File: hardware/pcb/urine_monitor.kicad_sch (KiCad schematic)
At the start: 26 parts, among them J1 LoadCell, J2 EInk_FPC, J3 USB-C_Power, Q1 SI2301, Q2 2N7002, SW1 USER_BTN, U1 RAK3172, U2 HX711, U3 TPS61220, U4 MIC5504-3.3

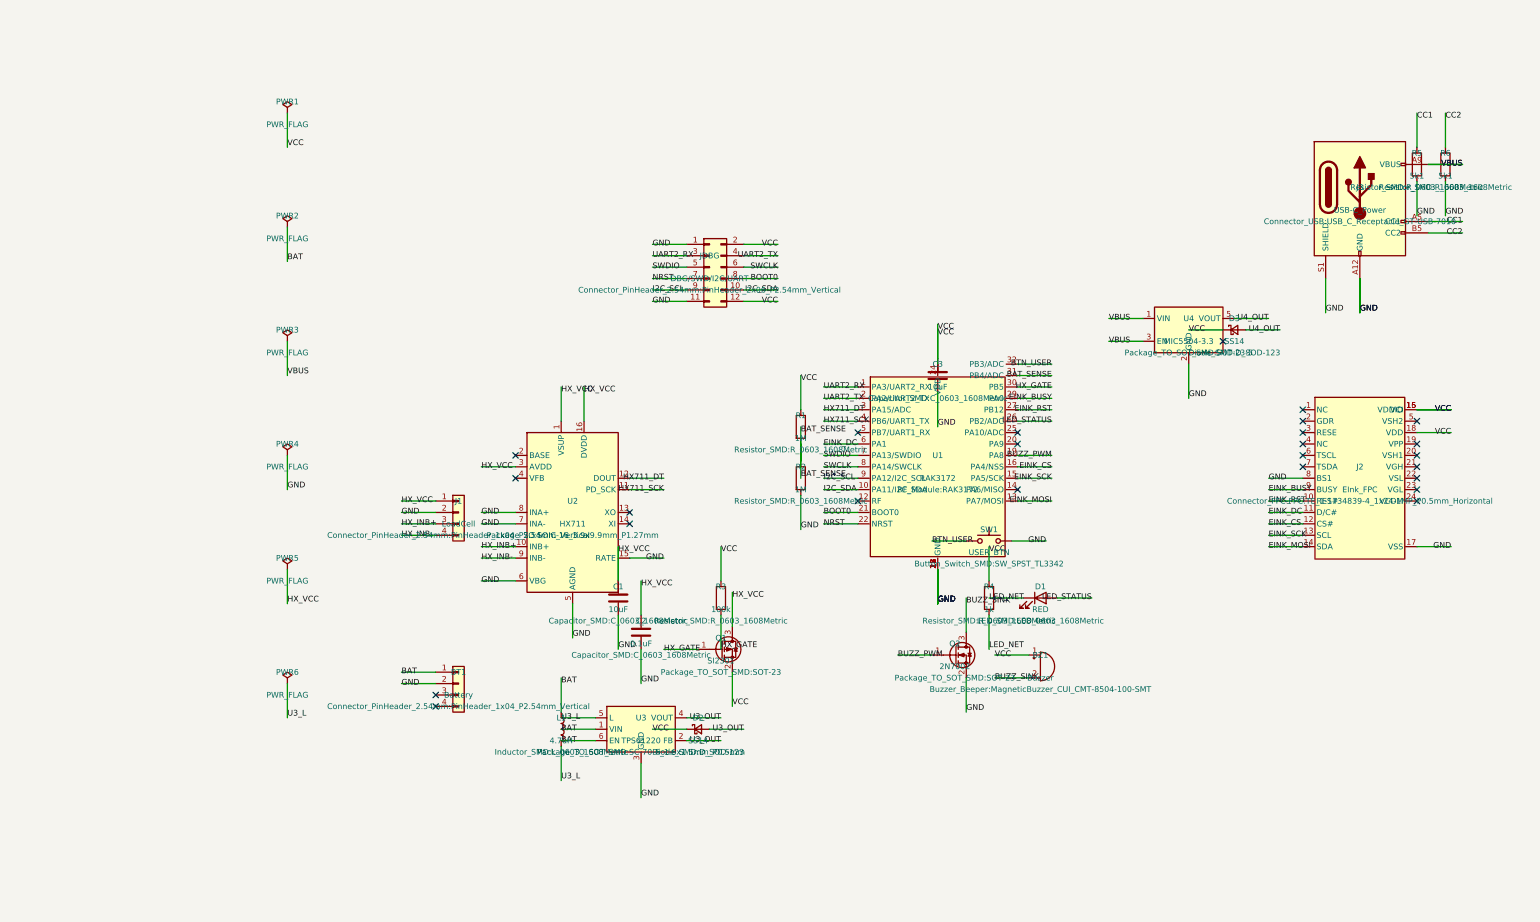
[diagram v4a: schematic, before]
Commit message: init
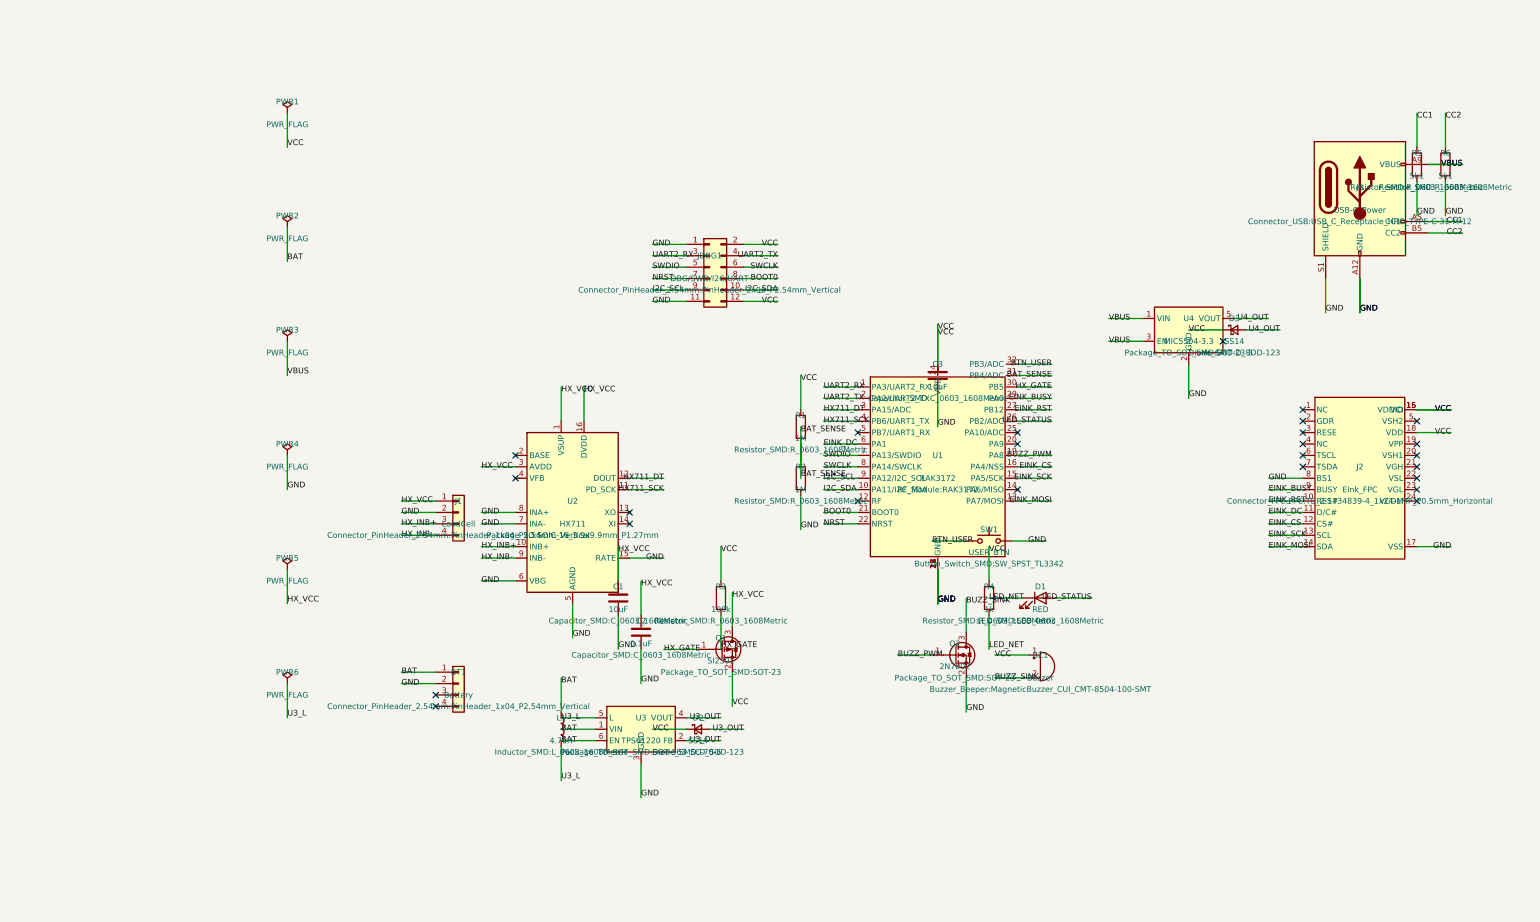
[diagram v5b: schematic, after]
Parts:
- removed JDBG: DBG/SWD/I2C/UART, Connector_PinHeader_2.54mm:PinHeader_2x06_P2.54mm_Vertical, symbol Connector_Generic:Conn_02x06_Odd_Even
- added JDBG1: DBG/SWD/I2C/UART, Connector_PinHeader_2.54mm:PinHeader_2x06_P2.54mm_Vertical, symbol Connector_Generic:Conn_02x06_Odd_Even
- J2: footprint Connector_FFC-FPC:TE_1-1734839-4_1x24-1MP_P0.5mm_Horizontal -> Connector_FFC-FPC:TE_2-1734839-4_1x24-1MP_P0.5mm_Horizontal
- J3: footprint Connector_USB:USB_C_Receptacle_GT-USB-7010 -> Connector_USB:USB_C_Receptacle_HRO_TYPE-C-31-M-12
- U3: footprint Package_TO_SOT_SMD:SC-70-6_1.6x1.5mm_P0.5mm -> Package_TO_SOT_SMD:SOT-363_SC-70-6
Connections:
- net BOOT0: now also JDBG1.8 (Pin_8)
- net GND: now also JDBG1.1 (Pin_1), JDBG1.11 (Pin_11)
- net I2C_SCL: now also JDBG1.9 (Pin_9)
- net I2C_SDA: now also JDBG1.10 (Pin_10)
- net NRST: now also JDBG1.7 (Pin_7)
- net SWCLK: now also JDBG1.6 (Pin_6)
- net SWDIO: now also JDBG1.5 (Pin_5)
- net UART2_RX: now also JDBG1.3 (Pin_3)
- net UART2_TX: now also JDBG1.4 (Pin_4)
- net VCC: now also JDBG1.12 (Pin_12), JDBG1.2 (Pin_2)
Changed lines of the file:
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@@
   (symbol (lib_id "Connector_Generic:Conn_02x06_Odd_Even") (at 119.38 59.69 0) (unit 1)
     (in_bom yes) (on_board yes)
-    (property "Reference" "JDBG" (id 0) (at 119.38 57.15 0)
+    (property "Reference" "JDBG1" (id 0) (at 119.38 57.15 0)
       (effects (font (size 1.27 1.27)))
     )
@@
       (effects (font (size 1.27 1.27)))
     )
-    (property "Footprint" "Connector_FFC-FPC:TE_1-1734839-4_1x24-1MP_P0.5mm_Horizontal" (id 2) (at 264.16 111.76 0) (effects (font (size 1.27 1.27))))
+    (property "Footprint" "Connector_FFC-FPC:TE_2-1734839-4_1x24-1MP_P0.5mm_Horizontal" (id 2) (at 264.16 111.76 0) (effects (font (size 1.27 1.27))))
   )
   (symbol (lib_id "Regulator_Switching:TPS61220DCK") (at 104.14 162.56 0) (unit 1)
@@
       (effects (font (size 1.27 1.27)))
     )
-    (property "Footprint" "Package_TO_SOT_SMD:SC-70-6_1.6x1.5mm_P0.5mm" (id 2) (at 104.14 167.64 0) (effects (font (size 1.27 1.27))))
+    (property "Footprint" "Package_TO_SOT_SMD:SOT-363_SC-70-6" (id 2) (at 104.14 167.64 0) (effects (font (size 1.27 1.27))))
   )
   (symbol (lib_id "Device:L") (at 86.36 162.56 0) (unit 1)
@@
       (effects (font (size 1.27 1.27)))
     )
-    (property "Footprint" "Connector_USB:USB_C_Receptacle_GT-USB-7010" (id 2) (at 264.16 49.53 0) (effects (font (size 1.27 1.27))))
+    (property "Footprint" "Connector_USB:USB_C_Receptacle_HRO_TYPE-C-31-M-12" (id 2) (at 264.16 49.53 0) (effects (font (size 1.27 1.27))))
   )
   (symbol (lib_id "Device:R") (at 276.86 36.83 0) (unit 1)
@@
     (property "Footprint" "Capacitor_SMD:C_0603_1608Metric" (id 2) (at 170.18 88.90 0) (effects (font (size 1.27 1.27))))
   )
-  (symbol (lib_id "Power:PWR_FLAG") (at 25.40 25.40 0) (unit 1)
+  (symbol (lib_id "Project_Lib:PWR_FLAG") (at 25.40 25.40 0) (unit 1)
     (in_bom yes) (on_board yes)
     (property "Reference" "PWR1" (id 0) (at 25.40 22.86 0)
@@
     )
   )
-  (symbol (lib_id "Power:PWR_FLAG") (at 25.40 50.80 0) (unit 1)
+  (symbol (lib_id "Project_Lib:PWR_FLAG") (at 25.40 50.80 0) (unit 1)
     (in_bom yes) (on_board yes)
     (property "Reference" "PWR2" (id 0) (at 25.40 48.26 0)
@@
     )
   )
-  (symbol (lib_id "Power:PWR_FLAG") (at 25.40 76.20 0) (unit 1)
+  (symbol (lib_id "Project_Lib:PWR_FLAG") (at 25.40 76.20 0) (unit 1)
     (in_bom yes) (on_board yes)
     (property "Reference" "PWR3" (id 0) (at 25.40 73.66 0)
@@
     )
   )
-  (symbol (lib_id "Power:PWR_FLAG") (at 25.40 101.60 0) (unit 1)
+  (symbol (lib_id "Project_Lib:PWR_FLAG") (at 25.40 101.60 0) (unit 1)
     (in_bom yes) (on_board yes)
     (property "Reference" "PWR4" (id 0) (at 25.40 99.06 0)
@@
     )
   )
-  (symbol (lib_id "Power:PWR_FLAG") (at 25.40 127.00 0) (unit 1)
+  (symbol (lib_id "Project_Lib:PWR_FLAG") (at 25.40 127.00 0) (unit 1)
     (in_bom yes) (on_board yes)
     (property "Reference" "PWR5" (id 0) (at 25.40 124.46 0)
@@
     )
   )
-  (symbol (lib_id "Power:PWR_FLAG") (at 25.40 152.40 0) (unit 1)
+  (symbol (lib_id "Project_Lib:PWR_FLAG") (at 25.40 152.40 0) (unit 1)
     (in_bom yes) (on_board yes)
     (property "Reference" "PWR6" (id 0) (at 25.40 149.86 0)
@@
     (path "/" (reference "U2") (unit 1))
     (path "/" (reference "J1") (unit 1))
-    (path "/" (reference "JDBG") (unit 1))
+    (path "/" (reference "JDBG1") (unit 1))
     (path "/" (reference "Q1") (unit 1))
     (path "/" (reference "R3") (unit 1))

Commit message: v0.0.2
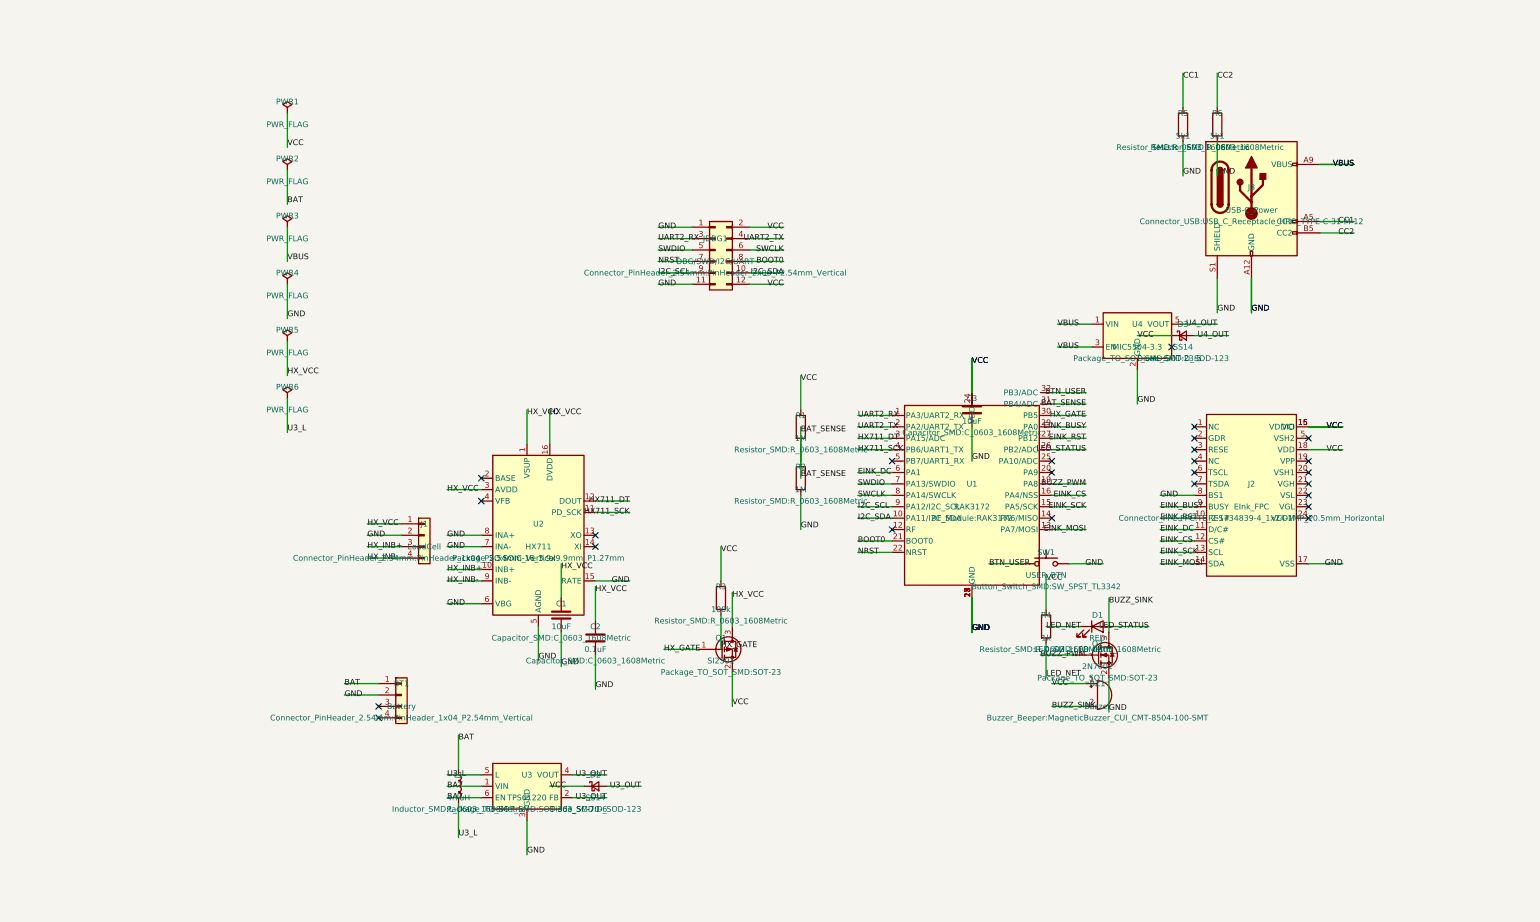
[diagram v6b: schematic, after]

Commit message: init
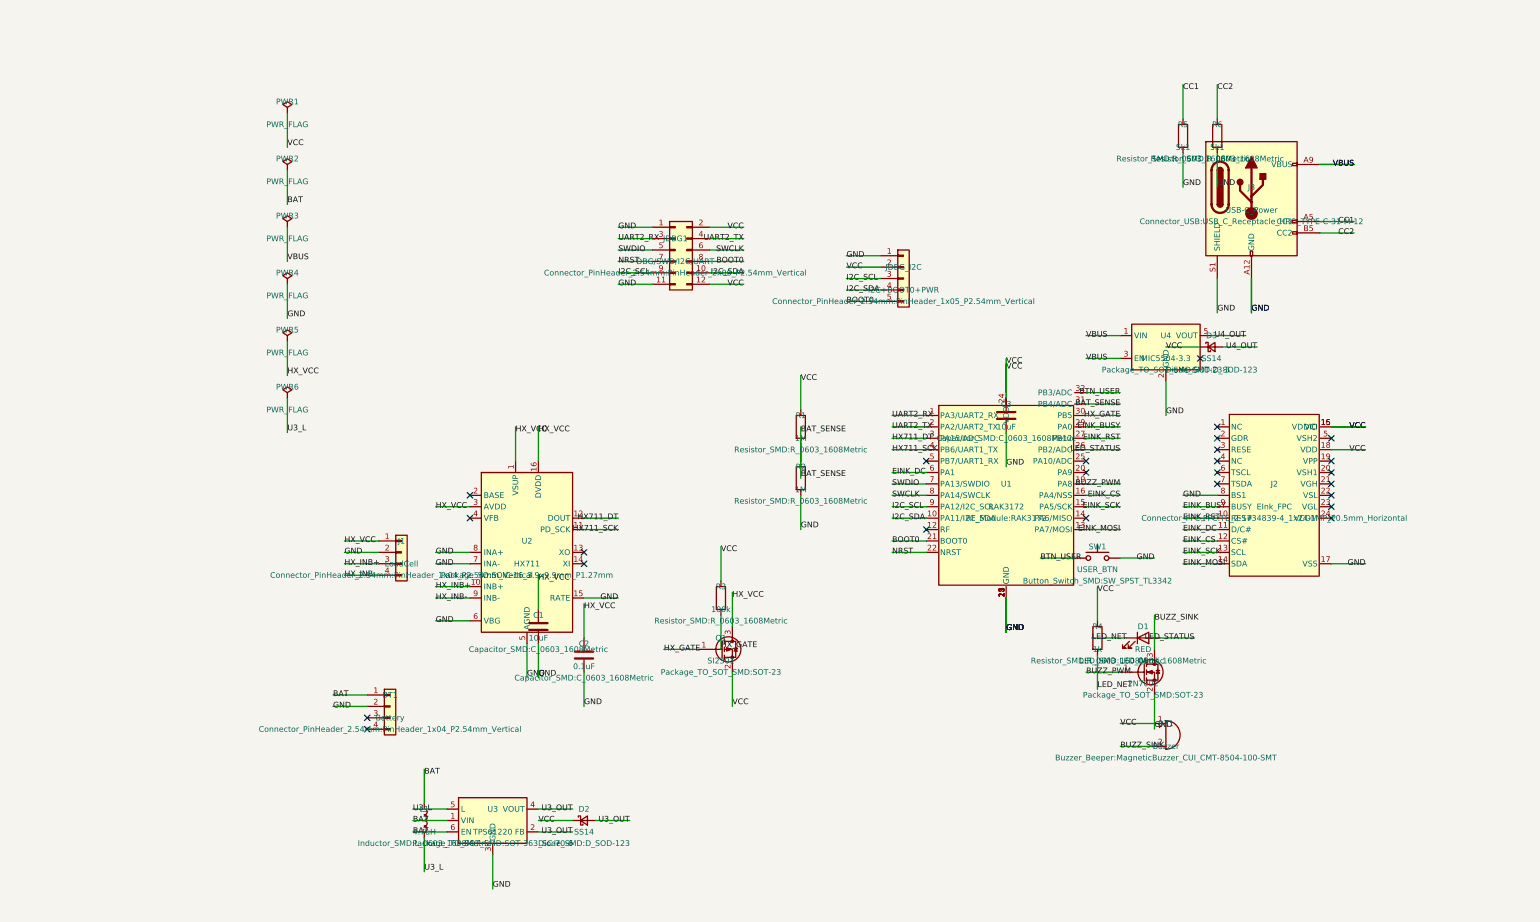
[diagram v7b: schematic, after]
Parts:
- added JDBG_I2C: I2C+BOOT0+PWR, Connector_PinHeader_2.54mm:PinHeader_1x05_P2.54mm_Vertical, symbol Connector_Generic:Conn_01x05
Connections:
- net BOOT0: now also JDBG_I2C.5 (Pin_5)
- net GND: now also JDBG_I2C.1 (Pin_1)
- net I2C_SCL: now also JDBG_I2C.3 (Pin_3)
- net I2C_SDA: now also JDBG_I2C.4 (Pin_4)
- net VCC: now also JDBG_I2C.2 (Pin_2)

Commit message: init
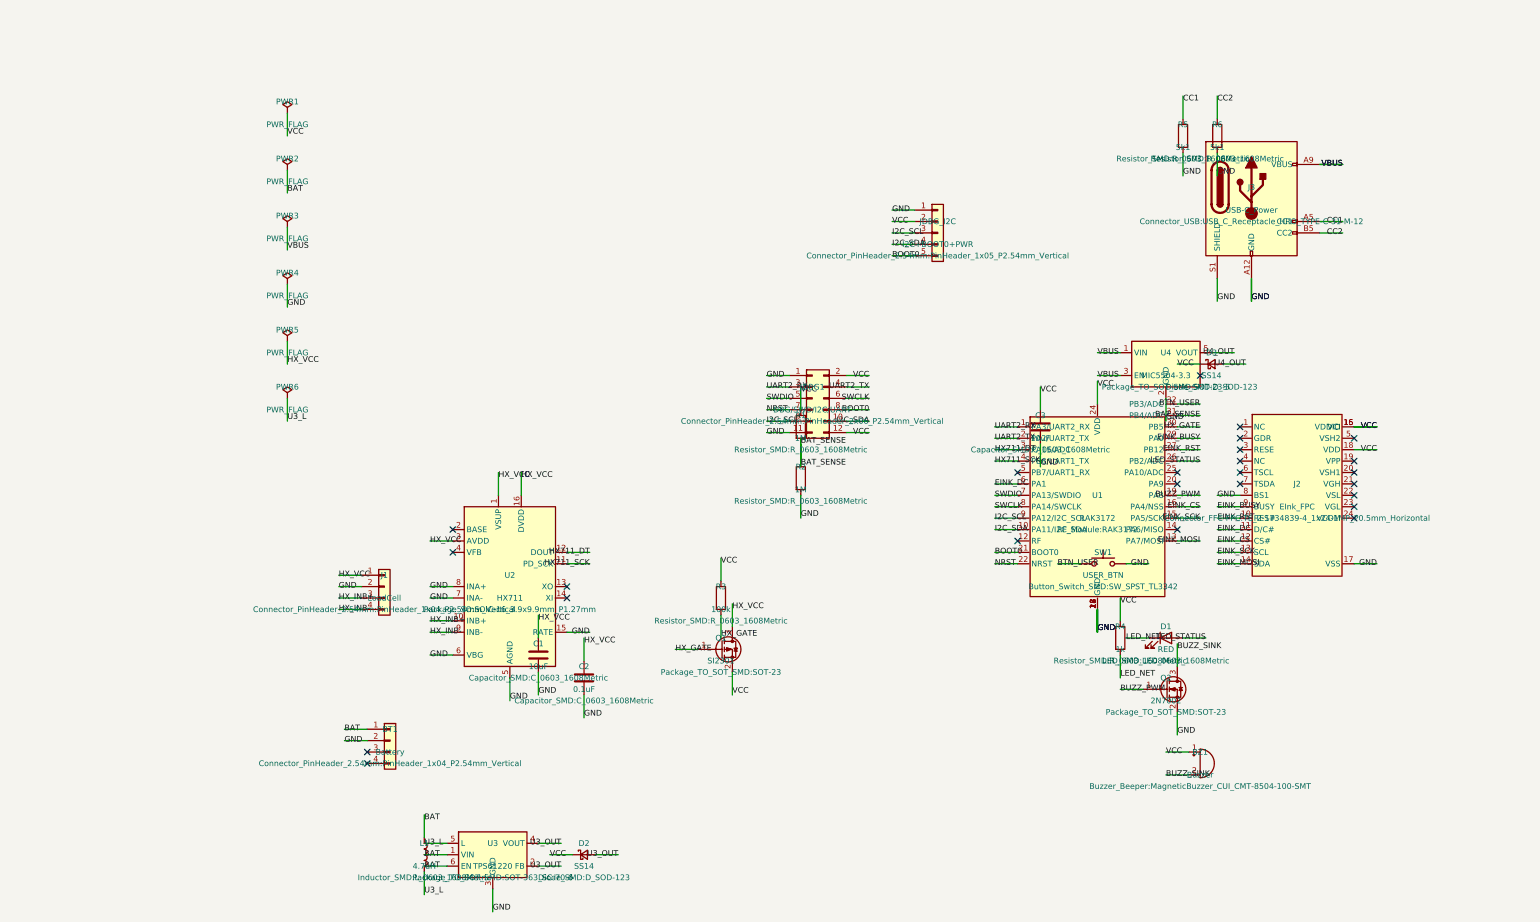
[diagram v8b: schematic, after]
